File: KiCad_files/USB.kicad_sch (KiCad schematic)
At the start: 4 parts, among them J1 USB_C_Receptacle_USB2.0_16P

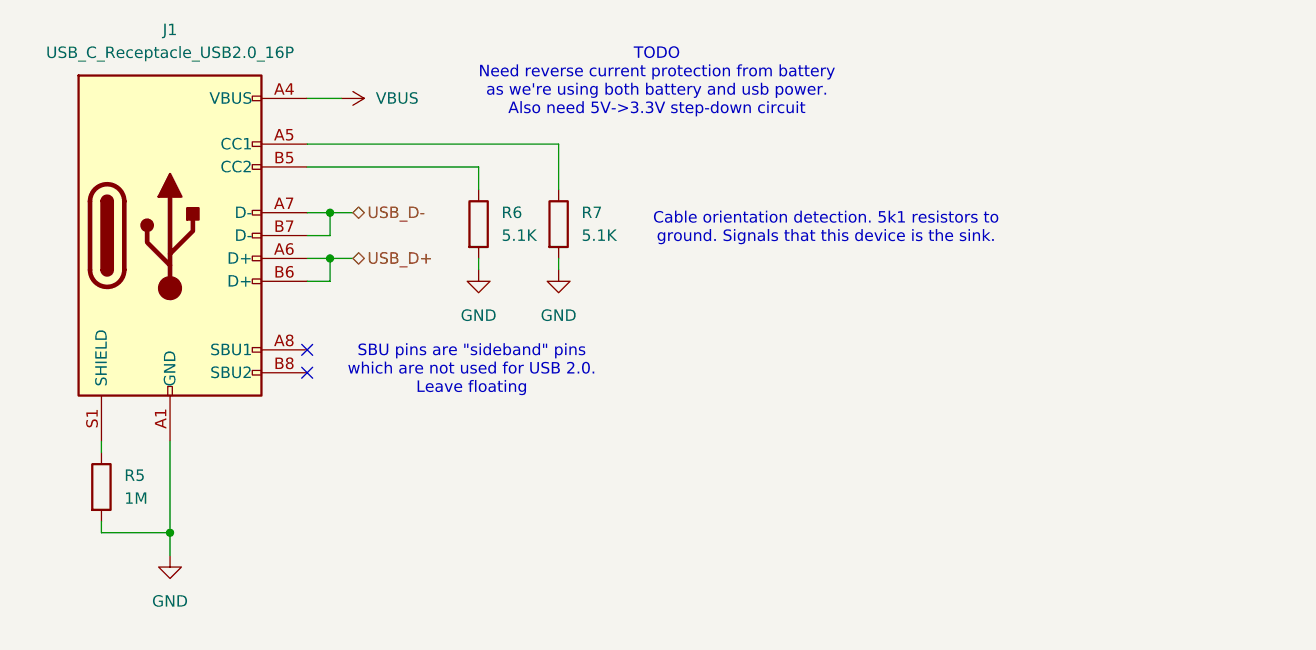
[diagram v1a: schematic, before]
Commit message: footprinttejä
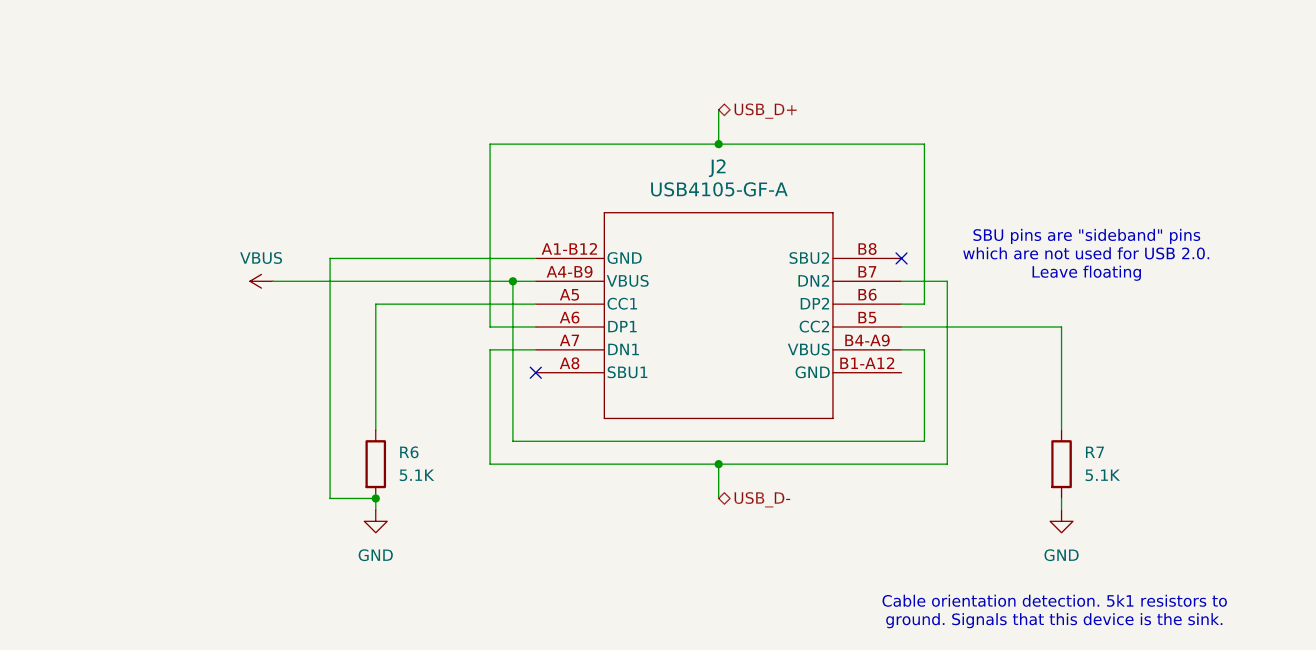
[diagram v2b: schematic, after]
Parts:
- removed J1: USB_C_Receptacle_USB2.0_16P, symbol Connector:USB_C_Receptacle_USB2.0_16P
- removed R5: 1M, symbol Device:R
- added J2: USB4105-GF-A, 1_project_library:USB4105_GCT, symbol 1_projektin osat:USB4105-GF-A
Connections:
- net GND: now also J2.A1-B12 (GND)
- net USB_D+: now also J2.A6 (DP1), J2.B6 (DP2)
- net USB_D-: now also J2.A7 (DN1), J2.B7 (DN2)
- net VBUS: now also J2.A4-B9 (VBUS), J2.B4-A9 (VBUS)
- net at R7.1: now also J2.B5 (CC2)
- net at R6.1: now also J2.A5 (CC1)
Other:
- note removed: "TODO Need reverse current protection from battery as we're using both battery and usb power. Also need 5V->3.3V step-down circuit"
- moved on the sheet: R6, R7
